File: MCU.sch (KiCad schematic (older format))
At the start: 54 parts, among them K1 G5Q-1A4 DC24, Q1 DMN3730U, U1 MCP9804, U19 TLP293-4, U3 ADM6320, U4 MCP2551-I-SN, U5 ESP32_DEVKITC, U6 MCP23008, U7 BQ32002, Y1 32K

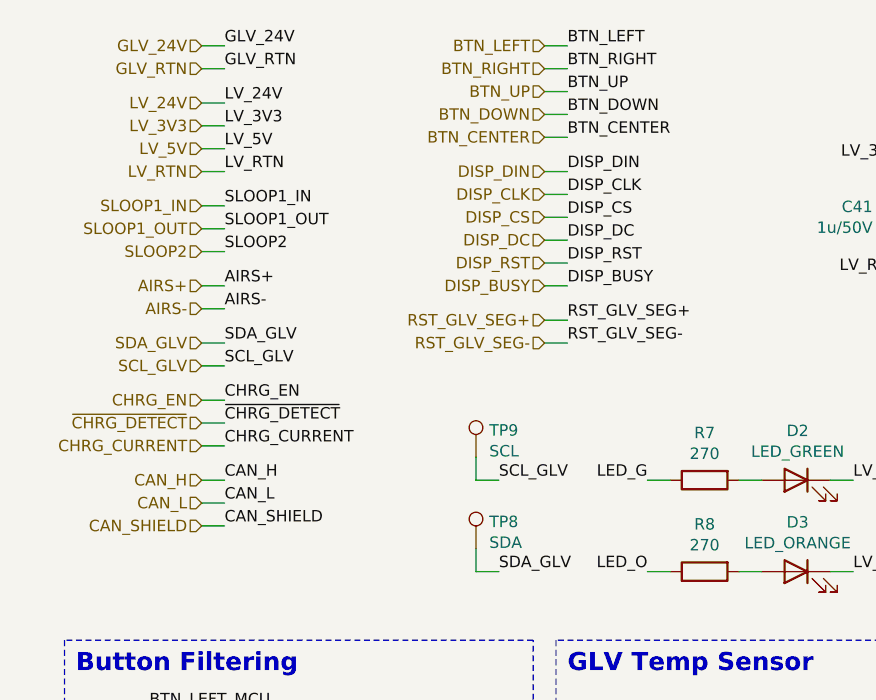
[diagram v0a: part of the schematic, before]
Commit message: Add files via upload
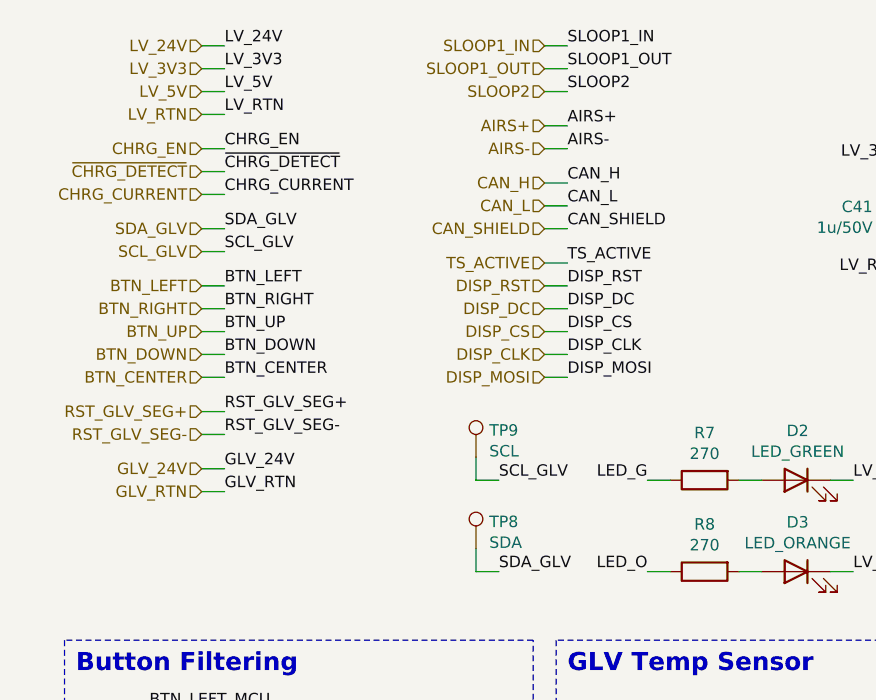
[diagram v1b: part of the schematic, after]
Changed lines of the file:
@@
 Text Label 5150 2150 2    50   ~ 0
 SLOOP_EN
-Text Label 1350 1350 0    50   ~ 0
-SLOOP1_IN
-Text Label 1350 1450 0    50   ~ 0
-SLOOP1_OUT
-Text Label 1350 1700 0    50   ~ 0
-AIRS+
-Text Label 1350 1800 0    50   ~ 0
-AIRS-
-Text HLabel 1250 1350 0    50   Input ~ 0
-SLOOP1_IN
-Text HLabel 1250 1450 0    50   Input ~ 0
-SLOOP1_OUT
-Text HLabel 1250 1700 0    50   Input ~ 0
-AIRS+
-Text HLabel 1250 1800 0    50   Input ~ 0
-AIRS-
-Wire Wire Line
-	1350 1800 1250 1800
-Wire Wire Line
-	1350 1700 1250 1700
-Wire Wire Line
-	1350 1450 1250 1450
-Wire Wire Line
-	1350 1350 1250 1350
 $Comp
 L Device:LED D2
@@
 Text Label 3200 2950 2    50   ~ 0
 LED_O
-Text HLabel 1250 1100 0    50   Input ~ 0
+Text HLabel 1250 850  0    50   Input ~ 0
 LV_5V
-Text HLabel 1250 1200 0    50   Input ~ 0
-LV_RTN
-Wire Wire Line
-	1250 1200 1350 1200
-Wire Wire Line
-	1250 1100 1350 1100
-Text Label 1350 1100 0    50   ~ 0
+Text HLabel 1250 950  0    50   Input ~ 0
+LV_RTN
+Wire Wire Line
+	1250 950  1350 950
+Wire Wire Line
+	1250 850  1350 850
+Text Label 1350 850  0    50   ~ 0
 LV_5V
-Text Label 1350 1200 0    50   ~ 0
+Text Label 1350 950  0    50   ~ 0
 LV_RTN
 Text Label 5150 950  2    50   ~ 0
 LV_3V3
-Text HLabel 1250 900  0    50   Input ~ 0
+Text HLabel 1250 650  0    50   Input ~ 0
 LV_24V
 Wire Wire Line
-	1250 900  1350 900
-Text Label 1350 900  0    50   ~ 0
+	1250 650  1350 650
+Text Label 1350 650  0    50   ~ 0
 LV_24V
 Text Label 4800 6200 0    50   ~ 0
 AIRS_STATUS
-Text Label 1350 2200 0    50   ~ 0
+Text Label 1350 1100 0    50   ~ 0
 CHRG_EN
-Text Label 1350 2300 0    50   ~ 0
+Text Label 1350 1200 0    50   ~ 0
 ~CHRG_DETECT
-Text Label 1350 2400 0    50   ~ 0
+Text Label 1350 1300 0    50   ~ 0
 CHRG_CURRENT
-Text Label 1350 1950 0    50   ~ 0
+Text Label 1350 1450 0    50   ~ 0
 SDA_GLV
-Text Label 1350 2050 0    50   ~ 0
+Text Label 1350 1550 0    50   ~ 0
 SCL_GLV
-Text HLabel 1250 2200 0    50   Input ~ 0
+Text HLabel 1250 1100 0    50   Input ~ 0
 CHRG_EN
-Text HLabel 1250 2300 0    50   Input ~ 0
+Text HLabel 1250 1200 0    50   Input ~ 0
 ~CHRG_DETECT
-Text HLabel 1250 2400 0    50   Input ~ 0
+Text HLabel 1250 1300 0    50   Input ~ 0
 CHRG_CURRENT
-Text HLabel 1250 1950 0    50   Input ~ 0
+Text HLabel 1250 1450 0    50   Input ~ 0
 SDA_GLV
-Text HLabel 1250 2050 0    50   Input ~ 0
+Text HLabel 1250 1550 0    50   Input ~ 0
 SCL_GLV
 Wire Wire Line
-	1350 2200 1250 2200
-Wire Wire Line
-	1250 2300 1350 2300
-Wire Wire Line
-	1350 2400 1250 2400
-Wire Wire Line
-	1250 1950 1350 1950
-Wire Wire Line
-	1350 2050 1250 2050
+	1350 1100 1250 1100
+Wire Wire Line
+	1250 1200 1350 1200
+Wire Wire Line
+	1350 1300 1250 1300
+Wire Wire Line
+	1250 1450 1350 1450
+Wire Wire Line
+	1350 1550 1250 1550
 Text Label 5150 1750 2    50   ~ 0
 CANTX
@@
 	0    -1   1    0
 $EndComp
-Text Label 1350 2550 0    50   ~ 0
+Text Label 2850 1250 0    50   ~ 0
 CAN_H
-Text Label 1350 2650 0    50   ~ 0
+Text Label 2850 1350 0    50   ~ 0
 CAN_L
-Text HLabel 1250 2550 0    50   Input ~ 0
+Text HLabel 2750 1250 0    50   Input ~ 0
 CAN_H
-Text HLabel 1250 2650 0    50   Input ~ 0
+Text HLabel 2750 1350 0    50   Input ~ 0
 CAN_L
 Wire Wire Line
-	1250 2550 1350 2550
-Wire Wire Line
-	1350 2650 1250 2650
+	2750 1250 2850 1250
+Wire Wire Line
+	2850 1350 2750 1350
 Text Label 5150 1050 2    50   ~ 0
 ~RESET
@@
 Wire Notes Line
 	2800 4950 2800 6450
-Text Label 2850 650  0    50   ~ 0
+Text Label 1350 1700 0    50   ~ 0
 BTN_LEFT
-Text Label 2850 750  0    50   ~ 0
+Text Label 1350 1800 0    50   ~ 0
 BTN_RIGHT
-Text Label 2850 850  0    50   ~ 0
+Text Label 1350 1900 0    50   ~ 0
 BTN_UP
-Text Label 2850 950  0    50   ~ 0
+Text Label 1350 2000 0    50   ~ 0
 BTN_DOWN
-Text Label 2850 1050 0    50   ~ 0
+Text Label 1350 2100 0    50   ~ 0
 BTN_CENTER
 Wire Wire Line
-	2750 1050 2850 1050
-Wire Wire Line
-	2850 950  2750 950
-Wire Wire Line
-	2750 850  2850 850
-Wire Wire Line
-	2850 750  2750 750
-Wire Wire Line
-	2750 650  2850 650
-Text Label 2850 1200 0    50   ~ 0
-DISP_DIN
-Text Label 2850 1300 0    50   ~ 0
+	1250 2100 1350 2100
+Wire Wire Line
+	1350 2000 1250 2000
+Wire Wire Line
+	1250 1900 1350 1900
+Wire Wire Line
+	1350 1800 1250 1800
+Wire Wire Line
+	1250 1700 1350 1700
+Text Label 2850 2100 0    50   ~ 0
+DISP_MOSI
+Text Label 2850 2000 0    50   ~ 0
 DISP_CLK
-Text Label 2850 1400 0    50   ~ 0
+Text Label 2850 1900 0    50   ~ 0
 DISP_CS
-Text Label 2850 1500 0    50   ~ 0
+Text Label 2850 1800 0    50   ~ 0
 DISP_DC
+Text Label 2850 1700 0    50   ~ 0
+DISP_RST
 Text Label 2850 1600 0    50   ~ 0
+TS_ACTIVE
+Text HLabel 2750 2100 0    50   Input ~ 0
+DISP_MOSI
+Text HLabel 2750 2000 0    50   Input ~ 0
+DISP_CLK
+Text HLabel 2750 1900 0    50   Input ~ 0
+DISP_CS
+Text HLabel 2750 1800 0    50   Input ~ 0
+DISP_DC
+Text HLabel 2750 1700 0    50   Input ~ 0
 DISP_RST
-Text Label 2850 1700 0    50   ~ 0
-DISP_BUSY
-Text HLabel 2750 1200 0    50   Input ~ 0
-DISP_DIN
-Text HLabel 2750 1300 0    50   Input ~ 0
-DISP_CLK
-Text HLabel 2750 1400 0    50   Input ~ 0
-DISP_CS
-Text HLabel 2750 1500 0    50   Input ~ 0
-DISP_DC
 Text HLabel 2750 1600 0    50   Input ~ 0
-DISP_RST
-Text HLabel 2750 1700 0    50   Input ~ 0
-DISP_BUSY
-Wire Wire Line
-	2750 1700 2850 1700
-Wire Wire Line
-	2850 1600 2750 1600
-Wire Wire Line
-	2750 1500 2850 1500
-Wire Wire Line
-	2850 1400 2750 1400
-Wire Wire Line
-	2750 1300 2850 1300
-Wire Wire Line
-	2850 1200 2750 1200
+TS_ACTIVE
+Wire Wire Line
+	2750 1600 2850 1600
+Wire Wire Line
+	2850 1700 2750 1700
+Wire Wire Line
+	2750 1800 2850 1800
+Wire Wire Line
+	2850 1900 2750 1900
+Wire Wire Line
+	2750 2000 2850 2000
+Wire Wire Line
+	2850 2100 2750 2100
 Text Label 3900 5500 2    50   ~ 0
 SDA_GLV
 Text Label 3900 5400 2    50   ~ 0
 SCL_GLV
-Text Label 1350 2750 0    50   ~ 0
+Text Label 2850 1450 0    50   ~ 0
 CAN_SHIELD
 Wire Wire Line
-	1350 2750 1250 2750
-Text HLabel 1250 2750 0    50   Input ~ 0
+	2850 1450 2750 1450
+Text HLabel 2750 1450 0    50   Input ~ 0
 CAN_SHIELD
 Wire Wire Line
@@
 Wire Wire Line
 	6950 2150 6850 2150
-Text Label 1350 1000 0    50   ~ 0
+Text Label 1350 750  0    50   ~ 0
 LV_3V3
-Text HLabel 1250 1000 0    50   Input ~ 0
+Text HLabel 1250 750  0    50   Input ~ 0
 LV_3V3
 Wire Wire Line
-	1250 1000 1350 1000
-Text HLabel 2750 1050 0    50   Input ~ 0
+	1250 750  1350 750
+Text HLabel 1250 2100 0    50   Input ~ 0
 BTN_CENTER
-Text HLabel 2750 950  0    50   Input ~ 0
+Text HLabel 1250 2000 0    50   Input ~ 0
 BTN_DOWN
-Text HLabel 2750 850  0    50   Input ~ 0
+Text HLabel 1250 1900 0    50   Input ~ 0
 BTN_UP
-Text HLabel 2750 750  0    50   Input ~ 0
+Text HLabel 1250 1800 0    50   Input ~ 0
 BTN_RIGHT
-Text HLabel 2750 650  0    50   Input ~ 0
+Text HLabel 1250 1700 0    50   Input ~ 0
 BTN_LEFT
 Text Label 6950 1850 0    50   ~ 0
@@
 Wire Wire Line
 	3000 7450 3100 7450
-Text HLabel 1250 1550 0    50   Input ~ 0
-SLOOP2
-Text Label 1350 1550 0    50   ~ 0
-SLOOP2
-Wire Wire Line
-	1350 1550 1250 1550
 Text Label 4800 6000 0    50   ~ 0
 SLOOP1_STATUS
@@
 Wire Wire Line
 	3900 6100 4000 6100
-Text HLabel 2750 1950 0    50   Input ~ 0
+Text HLabel 1250 2350 0    50   Input ~ 0
 RST_GLV_SEG-
 Wire Wire Line
-	2750 1950 2850 1950
+	1250 2350 1350 2350
 Text Label 4800 5800 0    50   ~ 0
 RST_GLV_SEG-
@@
 Text Label 4800 5700 0    50   ~ 0
 RST_GLV_SEG+
-Text Label 2850 1850 0    50   ~ 0
+Text Label 1350 2250 0    50   ~ 0
 RST_GLV_SEG+
-Text Label 2850 1950 0    50   ~ 0
+Text Label 1350 2350 0    50   ~ 0
 RST_GLV_SEG-
-Text HLabel 2750 1850 0    50   Input ~ 0
+Text HLabel 1250 2250 0    50   Input ~ 0
 RST_GLV_SEG+
 Wire Wire Line
-	2750 1850 2850 1850
+	1250 2250 1350 2250
 Wire Wire Line
 	8700 6050 8800 6050
@@
 Wire Wire Line
 	9600 4250 9650 4250
-Text HLabel 1250 650  0    50   Input ~ 0
+Text HLabel 1250 2500 0    50   Input ~ 0
 GLV_24V
 Wire Wire Line
-	1250 650  1350 650
-Text Label 1350 650  0    50   ~ 0
+	1250 2500 1350 2500
+Text Label 1350 2500 0    50   ~ 0
 GLV_24V
-Text Label 1350 750  0    50   ~ 0
+Text Label 1350 2600 0    50   ~ 0
 GLV_RTN
-Text HLabel 1250 750  0    50   Input ~ 0
+Text HLabel 1250 2600 0    50   Input ~ 0
 GLV_RTN
 Wire Wire Line
-	1250 750  1350 750
+	1250 2600 1350 2600
 Text Label 4800 5900 0    50   ~ 0
 GLV_STATUS
@@
 Text Notes 10300 1800 2    50   ~ 0
 ~~10uA draw
+Wire Wire Line
+	2850 850  2750 850
+Text Label 2850 850  0    50   ~ 0
+SLOOP2
+Text HLabel 2750 850  0    50   Input ~ 0
+SLOOP2
+Wire Wire Line
+	2850 650  2750 650
+Wire Wire Line
+	2850 750  2750 750
+Wire Wire Line
+	2850 1000 2750 1000
+Wire Wire Line
+	2850 1100 2750 1100
+Text HLabel 2750 1100 0    50   Input ~ 0
+AIRS-
+Text HLabel 2750 1000 0    50   Input ~ 0
+AIRS+
+Text HLabel 2750 750  0    50   Input ~ 0
+SLOOP1_OUT
+Text HLabel 2750 650  0    50   Input ~ 0
+SLOOP1_IN
+Text Label 2850 1100 0    50   ~ 0
+AIRS-
+Text Label 2850 1000 0    50   ~ 0
+AIRS+
+Text Label 2850 750  0    50   ~ 0
+SLOOP1_OUT
+Text Label 2850 650  0    50   ~ 0
+SLOOP1_IN
 $EndSCHEMATC
